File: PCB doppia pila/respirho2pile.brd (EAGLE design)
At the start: 40.1 x 25.1 mm, 29 parts, among them U1 ICM-20948, U2 1.8V/100mA, X2 32.768kHz

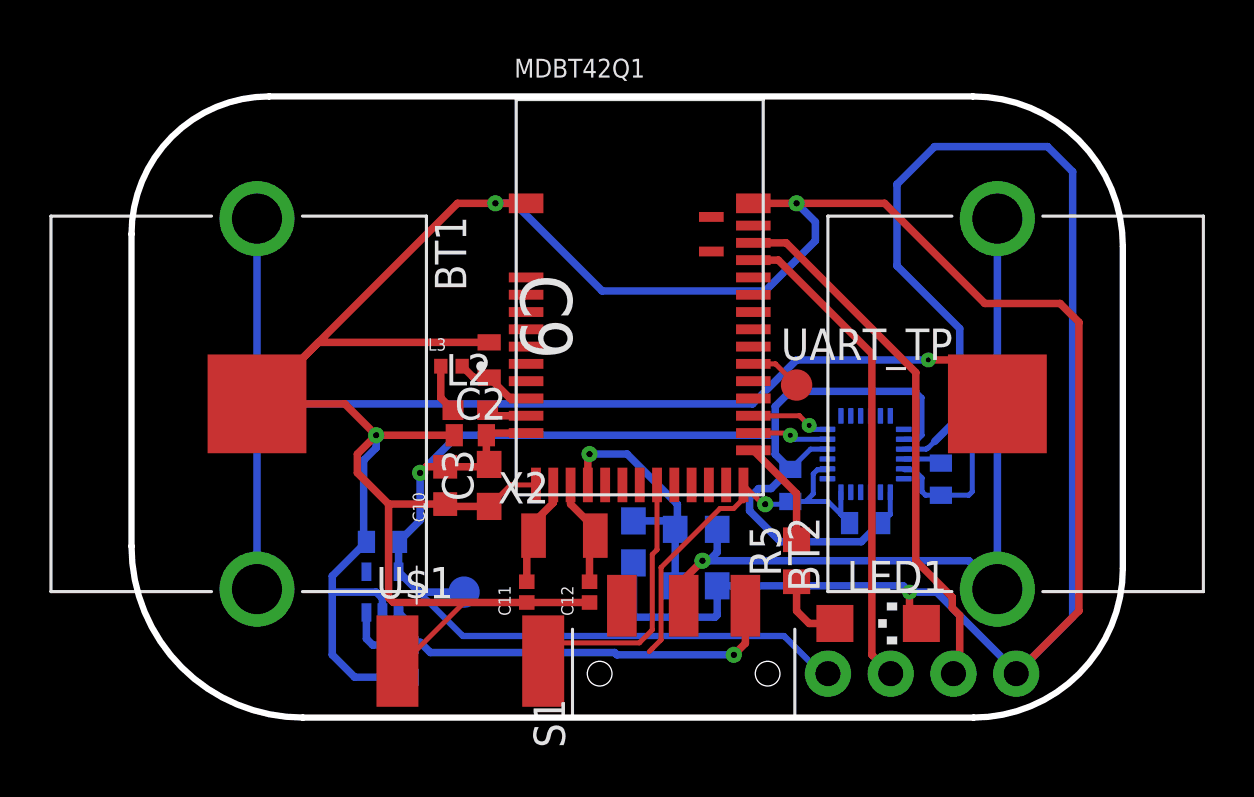
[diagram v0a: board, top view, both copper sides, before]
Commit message: Routing completo versione con 2 pile
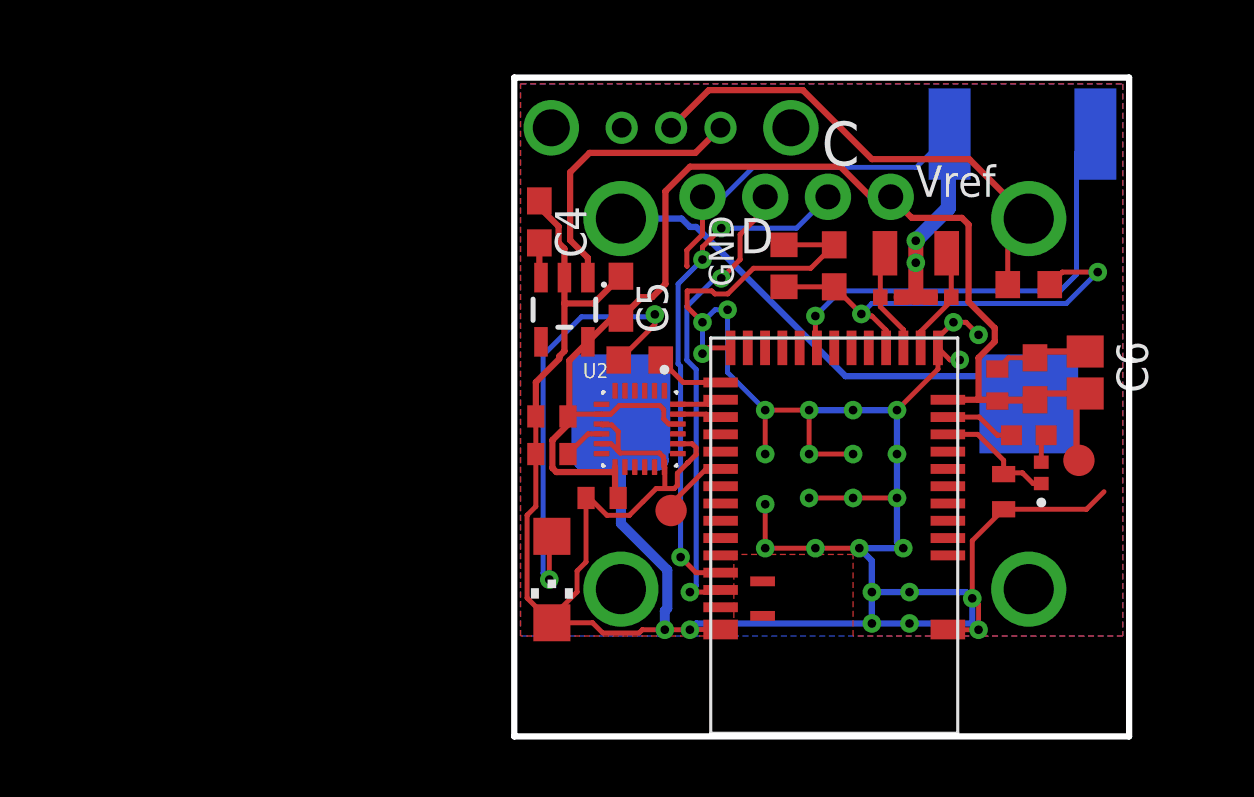
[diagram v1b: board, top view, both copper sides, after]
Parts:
- removed C10: 10uF, GRM188R61A106KE69J:CAPC1608X95N
- removed R5: 330, rcl:R0603
- removed S1: JS102011SAQN, JS102011SAQN:SW_JS102011SAQN
- removed U$1: KSS231GLFS, KSS231GLFS:KSS231GLFS
- removed X2: 32.768kHz, Nordic_nRF:XTAL_3215_N
- added C6: 10u, rcl:C2012
- added R3: 330, rcl:R0603
- added SW1: EG1213, Slide_switch:SW_EG1213
- added SW2: KSS231GLFS, KSS231GLFS:KSS231GLFS
- added X1: 32.768kHz, Nordic_nRF:XTAL_3215_N
- C4, C5: device rcl:C0402 -> rcl:C0603
- R1: value 850k -> 866k
- R2: value 800k -> 806k
- U2: value 1.8V/100mA -> AP2127K-1.8V; device SparkFun-IC-Power:SC70 -> TPS7A05:SOT23-5
- moved 1.8V_TP 25.5 mm to (38.4, 10.4), flipped to the top
- moved L3 24.3 mm to (36.8, 9.91), turned to 270 degrees
- moved J1 23.1 mm to (23.1, 21.1), turned to 0 degrees
- moved L2 22.6 mm to (36.3, 11.4), turned to 180 degrees
- moved C3 22.5 mm to (36.6, 13.7), turned to 270 degrees
- moved C9 21.5 mm to (35.3, 9.14), turned to 90 degrees
- moved C2 21.4 mm to (35.1, 13.5), turned to 270 degrees
- moved C11 20.6 mm to (32.8, 17.0), turned to 0 degrees
- moved C4 18.6 mm to (16.5, 20.1), flipped to the top
- moved C12 17.1 mm to (30.7, 17.0), turned to 180 degrees
- moved R2 16.7 mm to (36.3, 17.5), flipped to the top
- moved C15 15.8 mm to (17.0, 10.7), flipped to the top, turned to 0 degrees
- moved BT1 14.7 mm to (19.8, 12.7), flipped to the bottom, turned to 90 degrees
- moved C5 13.8 mm to (19.8, 17.0), flipped to the top, turned to 270 degrees
- moved C1 13.8 mm to (28.4, 18.3), flipped to the top, turned to 90 degrees
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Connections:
- net GND: now also C4.1, C5.1, C6.1, SW2.P$1; no longer C10.1, C4.2, C5.2, U$1.P$1
- net N$1: now also R3.1; no longer R5.1
- net N$5: now also R3.2; no longer R5.2
- net N$8: now also C4.2, SW1.3; no longer C4.1, S1.3
- net P0.00/XL1: now also X1.1; no longer X2.1
- net P0.01/XL2: now also X1.2; no longer X2.2
- net P06: now also SW2.P$2; no longer U$1.P$2
- net SCL: now also MDBT42Q1.27; no longer MDBT42Q1.26
- net SDA: now also MDBT42Q1.26; no longer MDBT42Q1.27
- net V+BATT: now also SW1.2; no longer S1.2
- net VDD: now also C5.2, C6.2; no longer C10.2, C5.1
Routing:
- net GND: track 211.4 -> 174.2 mm, vias 5 -> 32
- net N$6: track 46.4 -> 19.6 mm, vias 1 -> 0
- net VDD: track 73.7 -> 57.2 mm, vias 1 -> 0
- net N$1: track 2.94 -> 18.7 mm, vias 0 -> 2
- net V+BATT: track 31.0 -> 20.3 mm, vias 1 -> 0
- net P06: track 10.9 -> 18.6 mm, vias 0 -> 1
- net N$9: track 10.8 -> 18.0 mm, vias 1 -> 2
- net N$8: track 20.0 -> 12.8 mm, vias 1 -> 0
- net SWDIO: track 21.8 -> 19.0 mm, vias 0 -> 2
- net N$4: track 3.13 -> 4.98 mm
- net N$5: track 4.34 -> 2.80 mm
- net SDA: track 3.23 -> 1.80 mm, vias 1 -> 0
- net SCL: track 3.15 -> 1.78 mm, vias 1 -> 0
- net N$2: track 1.65 -> 2.88 mm
- net SWDCLK: track 19.6 -> 20.8 mm, vias 0 -> 3
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- added copper zone on layer 1, net GND
- added copper zone on layer 16, net GND
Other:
- board size 40.1 x 25.1 mm -> 24.9 x 26.7 mm
- board text added: "C"
- board text added: "D"
- board text added: "GND"
- board text added: "Vref"
